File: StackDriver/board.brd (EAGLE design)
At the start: 106.7 x 85.1 mm, 49 parts, among them IC1 LM741P, IC10 LM741P, IC11 LM741P, IC12 LM741P, IC13 LM741P, IC14 LM741P, IC15 LM741P, IC2 LM741P, IC3 LM741P, IC4 LM741P, IC5 LM741P, IC6 LM741P, IC7 LM741P, IC8 LM741P, IC9 LM741P

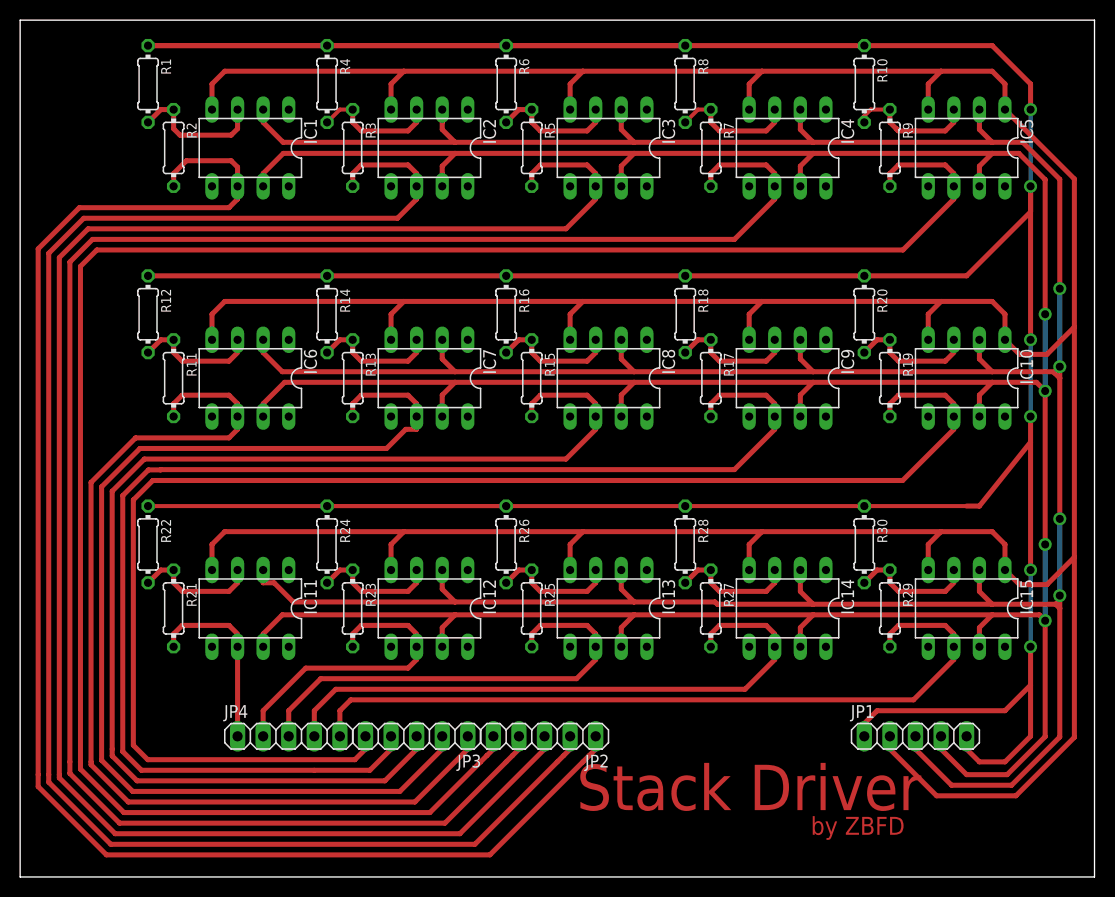
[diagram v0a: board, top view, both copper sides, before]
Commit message: debug
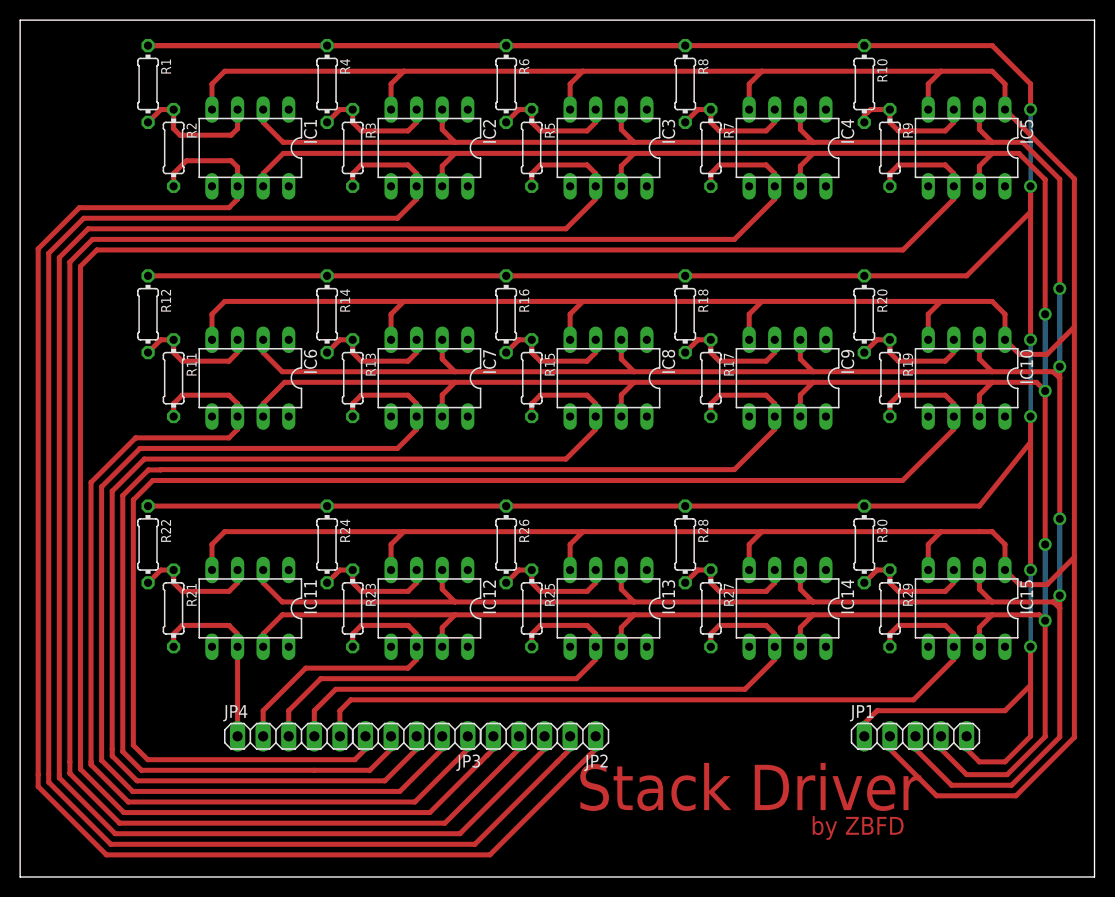
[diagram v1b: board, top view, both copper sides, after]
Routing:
- net GND: track 537.5 -> 519.7 mm
